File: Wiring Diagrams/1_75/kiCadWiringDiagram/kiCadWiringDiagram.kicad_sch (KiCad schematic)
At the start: 32 parts, among them J1 ESP32, J12 Speaker Connector, J2 Encoder Connector, J3 LED Connector, J4 Motor Connector, J5 12v Input 1, J6 12v Input 2, U1 LM2596S-5, U2 MC34063AD, U3 MMC5603NJ, U4 TMC6300-LA, U5 MCP23017_ML

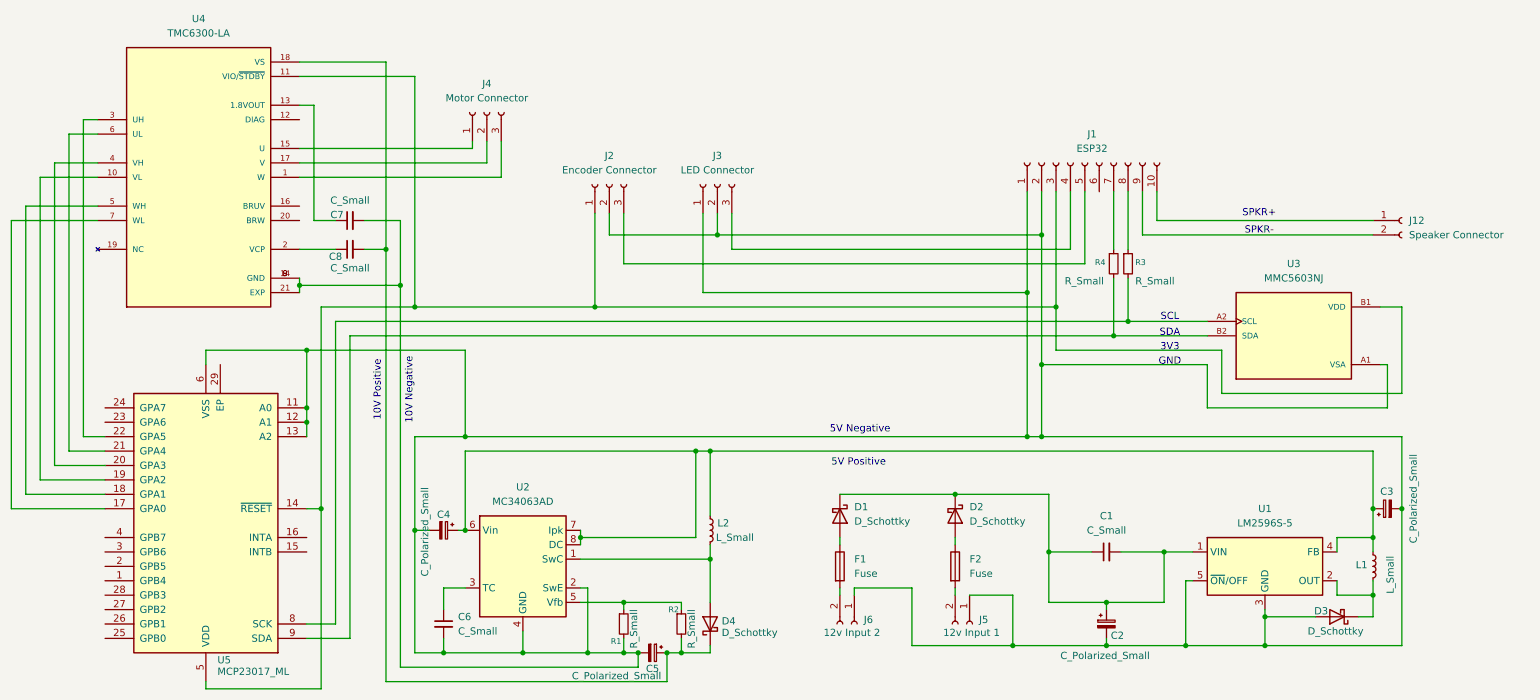
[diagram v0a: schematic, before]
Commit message: Completed footprints
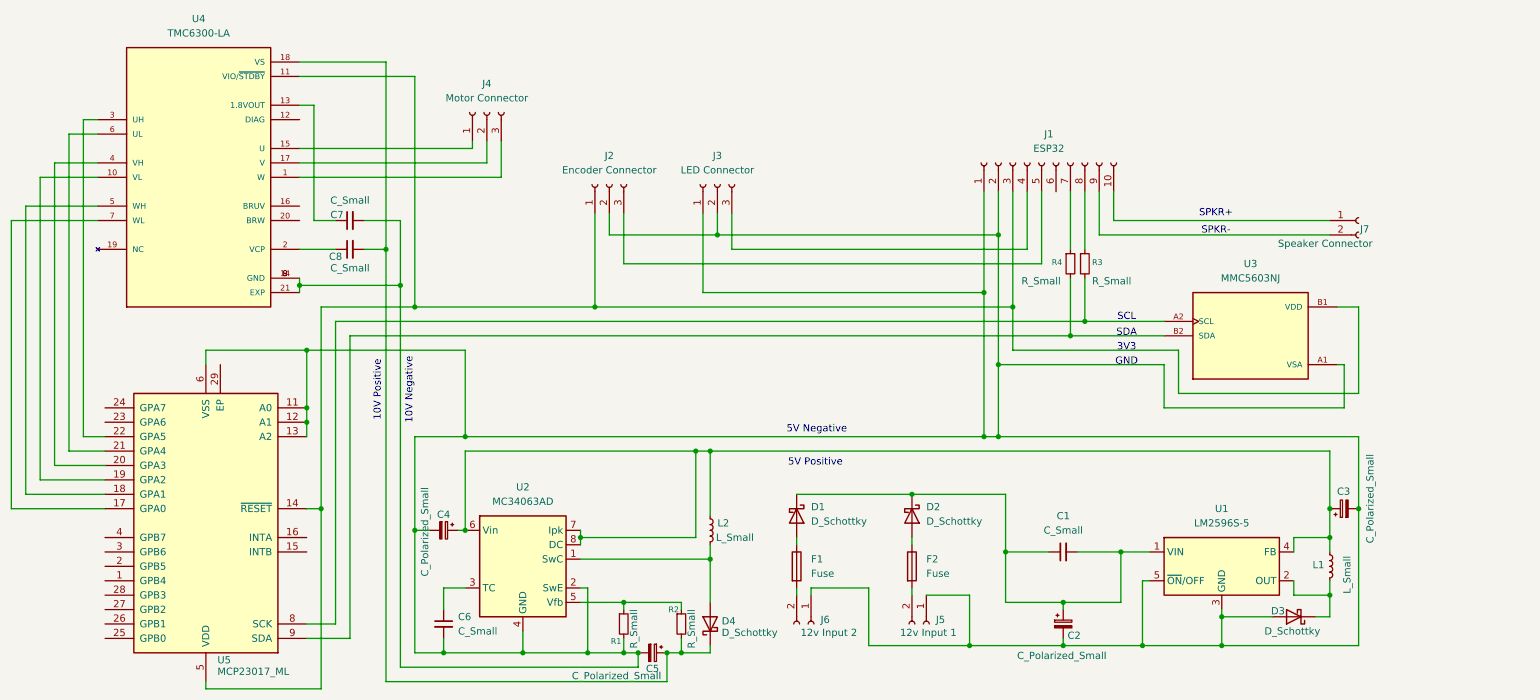
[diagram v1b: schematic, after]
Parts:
- C1, C6, C7, C8: footprint (none) -> Capacitor_SMD:C_0805_2012Metric
- C2, C3, C4, C5: footprint (none) -> Capacitor_SMD:CP_Elec_6.3x5.4
- D1, D2, D3, D4: footprint (none) -> Diode_SMD:D_SMA
- F1, F2: footprint (none) -> Fuse:Fuse_1206_3216Metric
- L1, L2: footprint (none) -> Inductor_SMD:L_7.3x7.3_H4.5
- R1, R2, R3, R4: footprint (none) -> Resistor_SMD:R_0805_2012Metric
- renumbered J12 to J7
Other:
- moved on the sheet: C1, C2, C3, D1, D2, D3, F1, F2, J1, J5, J6, J7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
